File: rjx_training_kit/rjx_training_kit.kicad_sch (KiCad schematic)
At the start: 19 parts, among them J1 Barrel_Jack_Switch, J2 ST-Link, J3 LD39200, SW1 SW_SPDT, U1 TLV76133DCY, U2 LD39200DPUR

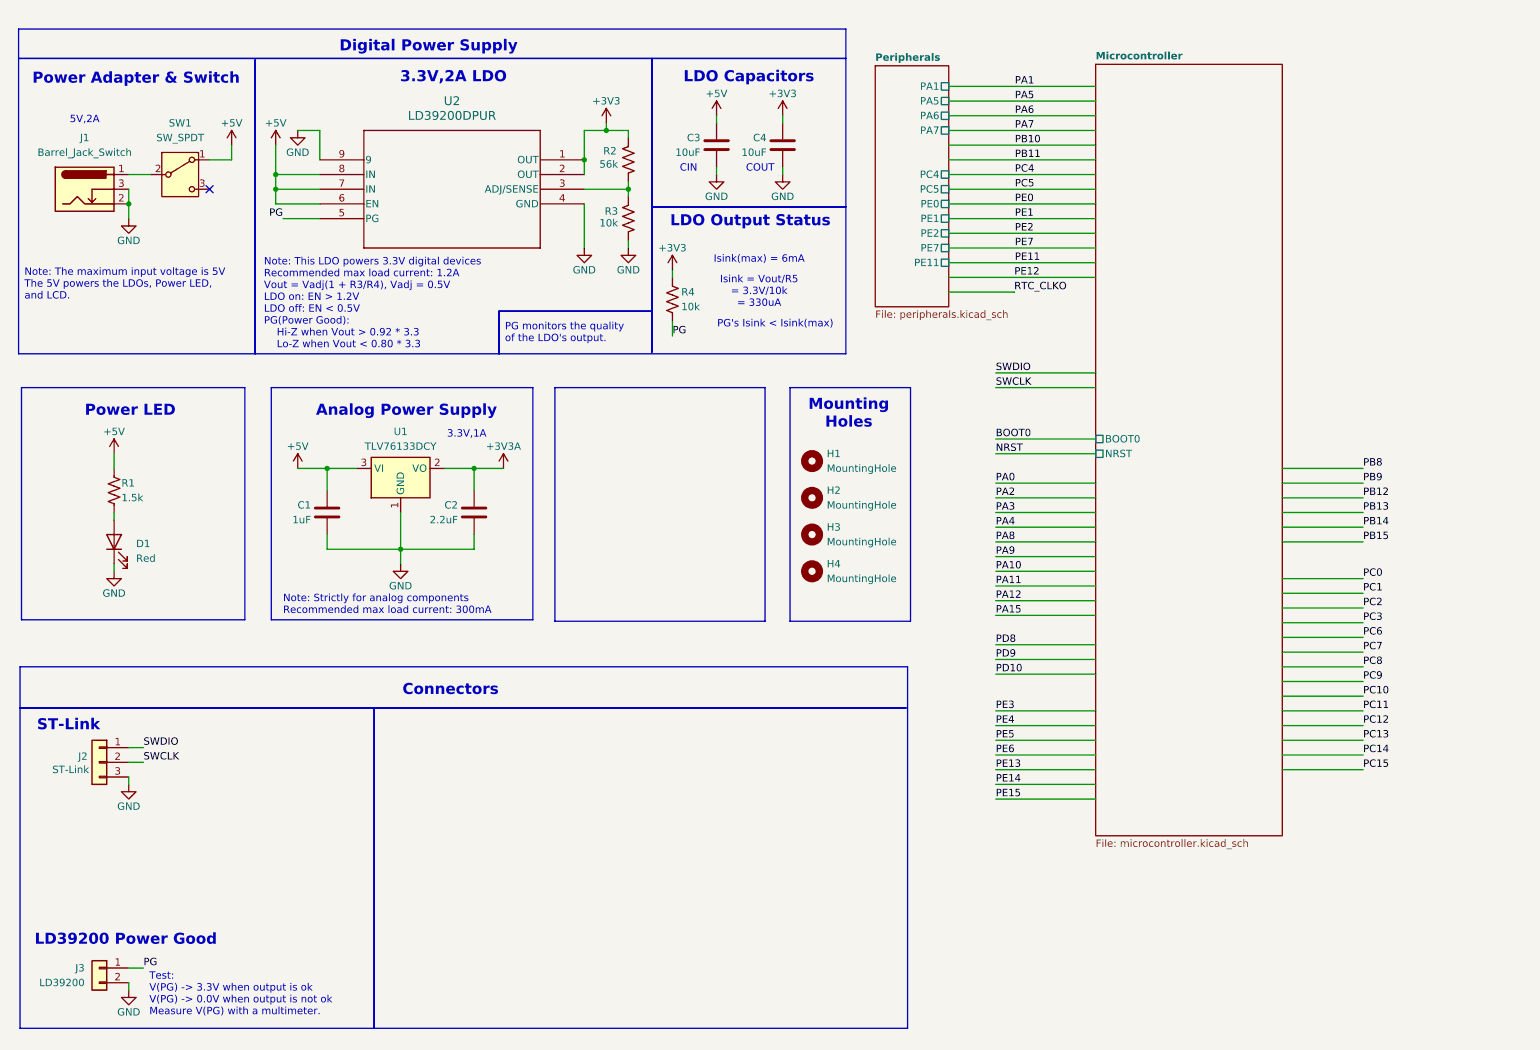
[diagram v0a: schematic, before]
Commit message: Update
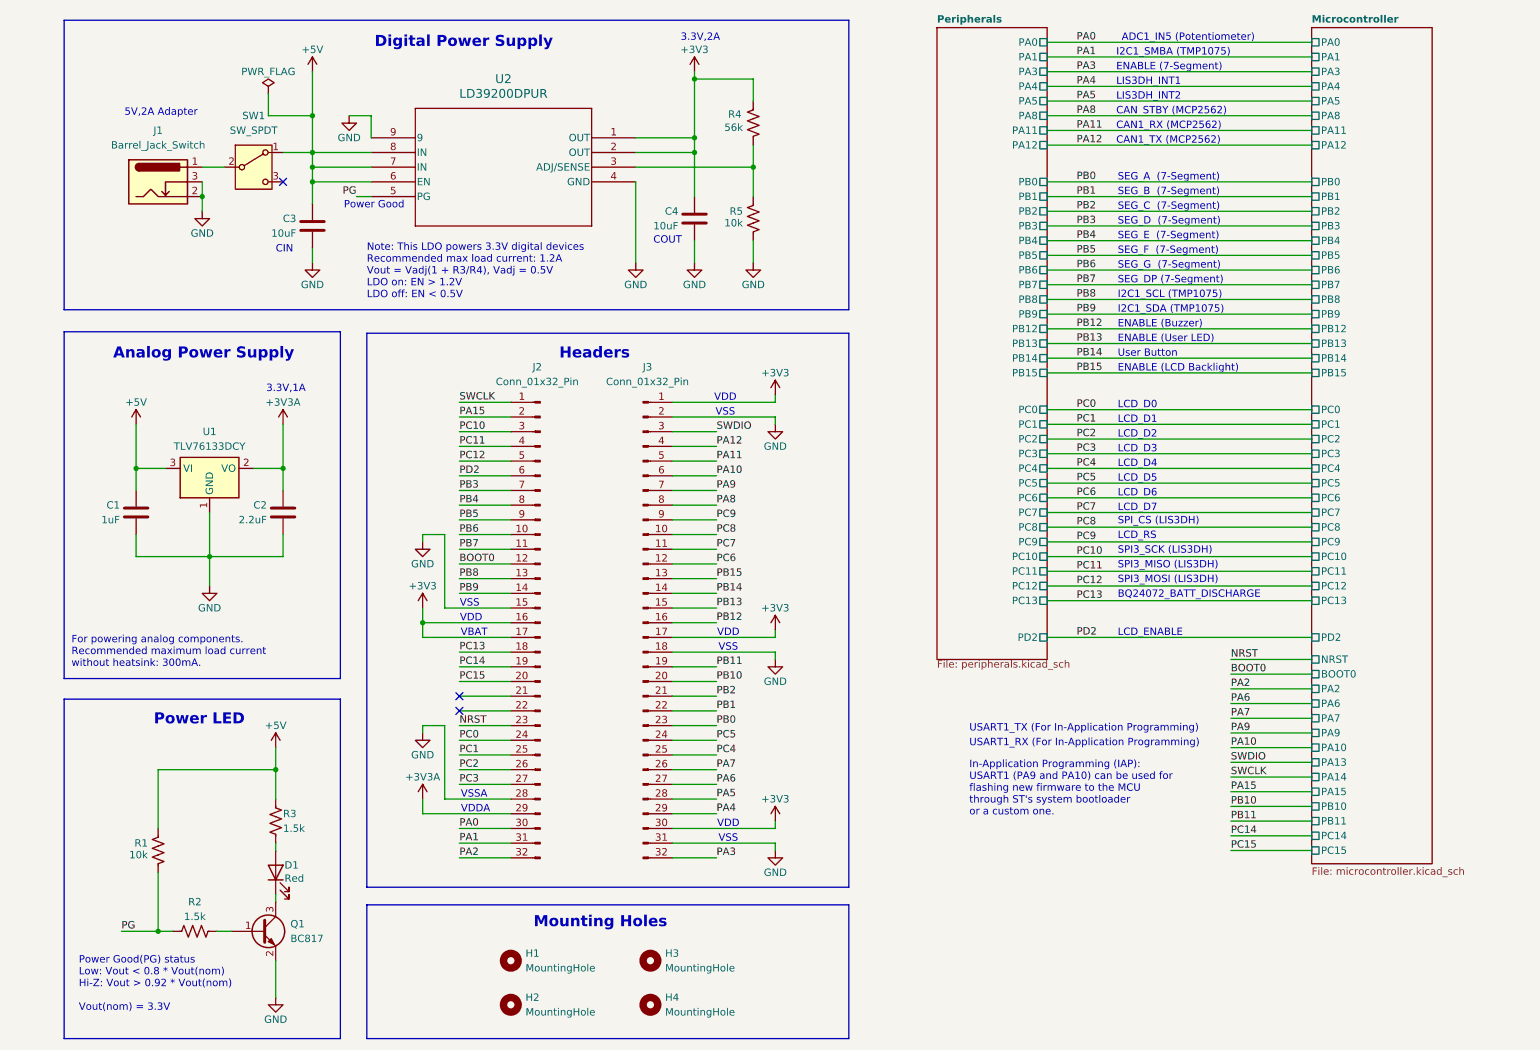
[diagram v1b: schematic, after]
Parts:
- removed J2: ST-Link, symbol Connector_Generic:Conn_01x03
- removed J3: LD39200, symbol Connector_Generic:Conn_01x02
- removed R4: 10k, symbol Device:R_US
- added J2, J3: Conn_01x32_Pin, symbol Connector:Conn_01x32_Pin
- added Q1: BC817, Package_TO_SOT_SMD:SOT-23, symbol Transistor_BJT:BC817
- added R1: 10k, symbol Device:R_US
- added R2: 1.5k, symbol Device:R_US
- U2: footprint LD39200:DFN-8-1EP_4x4mm_P0.8mm_EP2.3x3.24mm -> SON_0DPUR_STM
- renumbered H4 to H2, H2 to H3, H3 to H4, R1 to R3, R2 to R4, R3 to R5
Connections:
- net +3V3: now also J2.16 (Pin_16), J2.17 (Pin_17), J3.1 (Pin_1), J3.17 (Pin_17), J3.30 (Pin_30)
- net +3V3A: now also J2.29 (Pin_29)
- net +5V: now also R1.2
- net BOOT0: now also J2.12 (Pin_12)
- net GND: now also J2.15 (Pin_15), J2.28 (Pin_28), J3.18 (Pin_18), J3.2 (Pin_2), J3.31 (Pin_31), Q1.2 (E); no longer D1.1 (K)
- net NRST: now also J2.23 (Pin_23)
- net PA0: now also J2.30 (Pin_30)
- net PA1: now also J2.31 (Pin_31)
- net PA10: now also J3.6 (Pin_6)
- net PA11: now also J3.5 (Pin_5)
- net PA12: now also J3.4 (Pin_4)
- net PA15: now also J2.2 (Pin_2)
- net PA2: now also J2.32 (Pin_32)
- net PA3: now also J3.32 (Pin_32)
- net PA4: now also J3.29 (Pin_29)
- net PA5: now also J3.28 (Pin_28)
- net PA6: now also J3.27 (Pin_27)
- net PA7: now also J3.26 (Pin_26)
- net PA8: now also J3.8 (Pin_8)
- net PA9: now also J3.7 (Pin_7)
- net PB10: now also J3.20 (Pin_20)
- net PB11: now also J3.19 (Pin_19)
- net PB12: now also J3.16 (Pin_16)
- net PB13: now also J3.15 (Pin_15)
- net PB14: now also J3.14 (Pin_14)
- net PB15: now also J3.13 (Pin_13)
- net PB8: now also J2.13 (Pin_13)
- net PB9: now also J2.14 (Pin_14)
- net PC0: now also J2.24 (Pin_24)
- net PC1: now also J2.25 (Pin_25)
- net PC10: now also J2.3 (Pin_3)
- net PC11: now also J2.4 (Pin_4)
- net PC12: now also J2.5 (Pin_5)
- net PC13: now also J2.18 (Pin_18)
- net PC14: now also J2.19 (Pin_19)
- net PC15: now also J2.20 (Pin_20)
- net PC2: now also J2.26 (Pin_26)
- net PC3: now also J2.27 (Pin_27)
- net PC4: now also J3.25 (Pin_25)
- net PC5: now also J3.24 (Pin_24)
- net PC6: now also J3.12 (Pin_12)
- net PC7: now also J3.11 (Pin_11)
- net PC8: now also J3.10 (Pin_10)
- net PC9: now also J3.9 (Pin_9)
- net PG: now also R1.1, R2.1
- net SWCLK: now also J2.1 (Pin_1)
- net SWDIO: now also J3.3 (Pin_3)
- new net: Q1.1 (B), R2.2
- new net: D1.1 (K), Q1.3 (C)
- new net PB0: J3.23 (Pin_23)
- new net PB1: J3.22 (Pin_22)
- new net PB2: J3.21 (Pin_21)
- new net PB3: J2.7 (Pin_7)
- new net PB4: J2.8 (Pin_8)
- new net PB5: J2.9 (Pin_9)
- new net PB6: J2.10 (Pin_10)
- new net PB7: J2.11 (Pin_11)
- new net PD2: J2.6 (Pin_6)
- no-connect marks 1 -> 3
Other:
- sheet Microcontroller ports: added PA0, PA1, PA10, PA11, PA12, PA13, PA14, PA15, PA2, PA3, PA4, PA5, PA6, PA7, PA8, PA9, PB0, PB1, PB10, PB11, PB12, PB13, PB14, PB15, PB2, PB3, PB4, PB5, PB6, PB7, PB8, PB9, PC0, PC1, PC10, PC11, PC12, PC13, PC14, PC15, PC2, PC3, PC4, PC5, PC6, PC7, PC8, PC9, PD2; removed none
- sheet Peripherals ports: added PA0, PA11, PA12, PA3, PA4, PA8, PB0, PB1, PB12, PB13, PB14, PB15, PB2, PB3, PB4, PB5, PB6, PB7, PB8, PB9, PC0, PC1, PC10, PC11, PC12, PC13, PC2, PC3, PC6, PC7, PC8, PC9, PD2; removed PA6, PA7, PE0, PE1, PE11, PE2, PE7
- note added: "3.3V,2A"
- note added: "5V,2A Adapter"
- note added: "ADC1_IN5 (Potentiometer)"
- note added: "BQ24072_BATT_DISCHARGE"
- note added: "CAN1_RX (MCP2562)"
- note added: "CAN1_TX (MCP2562)"
- note added: "CAN_STBY (MCP2562)"
- note added: "ENABLE (7-Segment)"
- note added: "ENABLE (Buzzer)"
- note added: "ENABLE (LCD Backlight)"
- note added: "ENABLE (User LED)"
- note added: "For powering analog components. Recommended maximum load current without heatsink: 300mA."
- note added: "Headers"
- note added: "I2C1_SCL (TMP1075)"
- note added: "I2C1_SDA (TMP1075)"
- note added: "I2C1_SMBA (TMP1075)"
- note added: "In-Application Programming (IAP): USART1 (PA9 and PA10) can be used for flashing new firmware to the MCU through ST's system bootloader or a custom one."
- note added: "LCD_D0"
- note added: "LCD_D1"
- note added: "LCD_D2"
- note added: "LCD_D3"
- note added: "LCD_D4"
- note added: "LCD_D5"
- note added: "LCD_D6"
- note added: "LCD_D7"
- note added: "LCD_ENABLE"
- note added: "LCD_RS"
- note added: "LIS3DH_INT1"
- note added: "LIS3DH_INT2"
- note added: "Note: This LDO powers 3.3V digital devices Recommended max load current: 1.2A Vout = Vadj(1 + R3/R4), Vadj = 0.5V LDO on: EN > 1.2V LDO off: EN < 0.5V"
- note added: "Power Good"
- note added: "Power Good(PG) status Low: Vout < 0.8 * Vout(nom) Hi-Z: Vout > 0.92 * Vout(nom) Vout(nom) = 3.3V"
- note added: "SEG_A (7-Segment)"
- note added: "SEG_B (7-Segment)"
- note added: "SEG_C (7-Segment)"
- note added: "SEG_D (7-Segment)"
- note added: "SEG_DP (7-Segment)"
- note added: "SEG_E (7-Segment)"
- note added: "SEG_F (7-Segment)"
- note added: "SEG_G (7-Segment)"
- note added: "SPI3_MISO (LIS3DH)"
- note added: "SPI3_MOSI (LIS3DH)"
- note added: "SPI3_SCK (LIS3DH)"
- note added: "SPI_CS (LIS3DH)"
- note added: "USART1_RX (For In-Application Programming)"
- note added: "USART1_TX (For In-Application Programming)"
- note added: "User Button"
- note added: "VBAT"
- note added: "VDD"
- note added: "VDDA"
- note added: "VSS"
- note added: "VSSA"
- note removed: "3.3V,2A LDO"
- note removed: "5V,2A"
- note removed: "Connectors"
- note removed: "Isink = Vout/R5 = 3.3V/10k = 330uA"
- note removed: "Isink(max) = 6mA"
- note removed: "LD39200 Power Good"
- note removed: "LDO Capacitors"
- note removed: "LDO Output Status"
- note removed: "Note: Strictly for analog components Recommended max load current: 300mA"
- note removed: "Note: The maximum input voltage is 5V The 5V powers the LDOs, Power LED, and LCD."
- note removed: "Note: This LDO powers 3.3V digital devices Recommended max load current: 1.2A Vout = Vadj(1 + R3/R4), Vadj = 0.5V LDO on: EN > 1.2V LDO off: EN < 0.5V PG(Power Good): Hi-Z when Vout > 0.92 * 3.3 Lo-Z when Vout < 0.80 * 3.3"
- note removed: "PG monitors the quality of the LDO's output."
- note removed: "PG's Isink < Isink(max)"
- note removed: "Power Adapter & Switch"
- note removed: "ST-Link"
- note removed: "Test: V(PG) -> 3.3V when output is ok V(PG) -> 0.0V when output is not ok Measure V(PG) with a multimeter."
- moved on the sheet: C3, C4, D1, H1, H2, H3, H4, J1, R3, R4, R5, SW1
